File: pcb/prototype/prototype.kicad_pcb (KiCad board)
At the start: 2 copper layers, 39 parts, among them J1 GS2, J10 Conn_01x14, J11 Conn_01x14, J12 Conn_01x08, J13 Conn_01x08, J2 GS2, J3 GS2, J4 GS2, J5 GS2, J6 GS2, J7 GS2, J8 GS2, J9 Conn_01x14

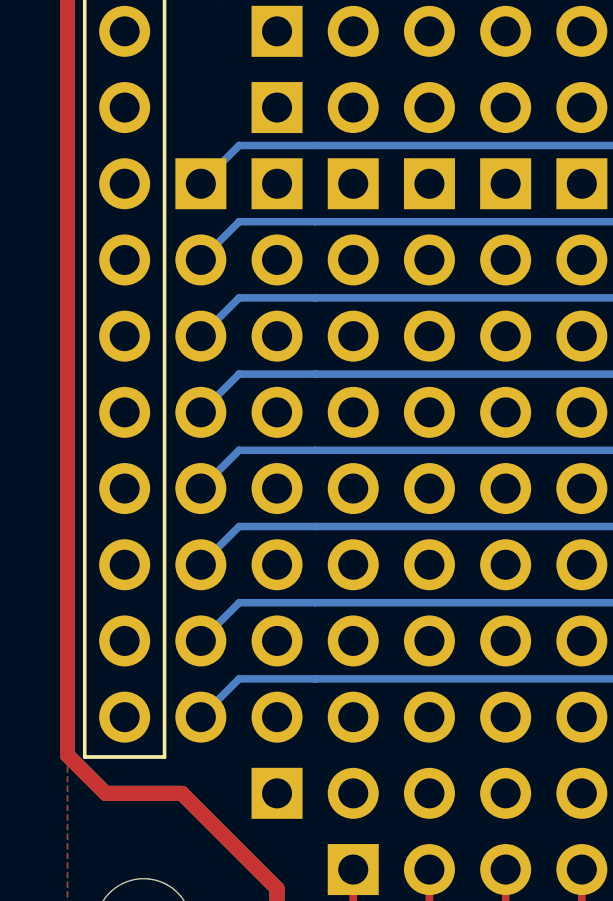
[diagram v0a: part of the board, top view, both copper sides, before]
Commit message: Ready for the second batch of PCBs to be printed.
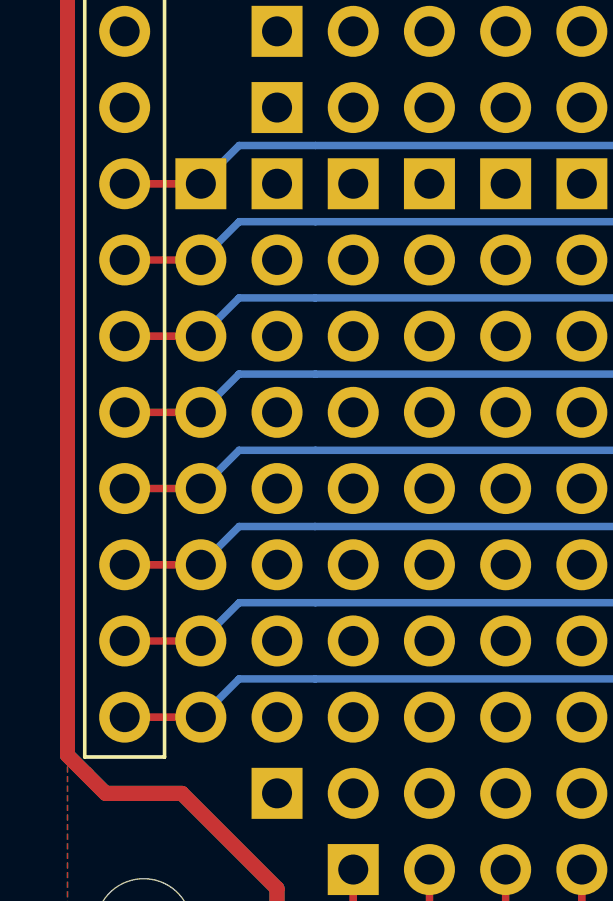
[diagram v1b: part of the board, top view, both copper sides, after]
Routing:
- net /L7: track 42.4 -> 45.0 mm
- net /L6: track 38.6 -> 41.2 mm
- net /L5: track 42.4 -> 45.0 mm
- net /L4: track 38.6 -> 41.2 mm
- net /L3: track 42.4 -> 45.0 mm
- net /L2: track 38.6 -> 41.2 mm
- net /L1: track 42.4 -> 45.0 mm
- net /L0: track 38.6 -> 41.2 mm
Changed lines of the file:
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@@
   (general
     (links 99)
-    (no_connects 8)
-    (area 123.19 81.915 172.720001 131.71)
+    (no_connects 0)
+    (area 123.19 81.915 172.720001 131.445001)
     (thickness 1.6)
     (drawings 15)
-    (tracks 151)
+    (tracks 159)
     (zones 0)
     (modules 39)
@@
   (segment (start 127 92.075) (end 128.905 90.17) (width 0.5) (layer F.Cu) (net 1))
   (segment (start 128.905 90.17) (end 131.445 90.17) (width 0.5) (layer F.Cu) (net 1))
+  (segment (start 126.365 102.87) (end 128.905 102.87) (width 0.25) (layer F.Cu) (net 3))
   (segment (start 167.005 101.595) (end 132.72 101.595) (width 0.25) (layer B.Cu) (net 3))
   (segment (start 132.72 101.595) (end 130.18 101.595) (width 0.25) (layer B.Cu) (net 3))
   (segment (start 130.18 101.595) (end 128.905 102.87) (width 0.25) (layer B.Cu) (net 3))
+  (segment (start 126.365 105.41) (end 128.905 105.41) (width 0.25) (layer F.Cu) (net 4))
   (segment (start 170.815 104.135) (end 132.72 104.135) (width 0.25) (layer B.Cu) (net 4))
   (segment (start 132.72 104.135) (end 130.18 104.135) (width 0.25) (layer B.Cu) (net 4))
   (segment (start 130.18 104.135) (end 128.905 105.41) (width 0.25) (layer B.Cu) (net 4))
+  (segment (start 126.365 107.95) (end 128.905 107.95) (width 0.25) (layer F.Cu) (net 5))
   (segment (start 132.715 106.675) (end 130.18 106.675) (width 0.25) (layer B.Cu) (net 5))
   (segment (start 130.18 106.675) (end 128.905 107.95) (width 0.25) (layer B.Cu) (net 5))
   (segment (start 167.005 106.675) (end 132.715 106.675) (width 0.25) (layer B.Cu) (net 5))
+  (segment (start 126.365 110.49) (end 128.905 110.49) (width 0.25) (layer F.Cu) (net 6))
   (segment (start 132.72 109.215) (end 130.18 109.215) (width 0.25) (layer B.Cu) (net 6))
   (segment (start 130.175 109.22) (end 128.905 110.49) (width 0.25) (layer B.Cu) (net 6))
   (segment (start 130.18 109.215) (end 130.175 109.22) (width 0.25) (layer B.Cu) (net 6))
   (segment (start 170.815 109.215) (end 132.72 109.215) (width 0.25) (layer B.Cu) (net 6))
+  (segment (start 126.365 113.03) (end 128.905 113.03) (width 0.25) (layer F.Cu) (net 7))
   (segment (start 132.72 111.755) (end 130.18 111.755) (width 0.25) (layer B.Cu) (net 7))
   (segment (start 130.18 111.755) (end 128.905 113.03) (width 0.25) (layer B.Cu) (net 7))
   (segment (start 167.005 111.755) (end 132.72 111.755) (width 0.25) (layer B.Cu) (net 7))
+  (segment (start 126.365 115.57) (end 128.905 115.57) (width 0.25) (layer F.Cu) (net 8))
   (segment (start 132.715 114.295) (end 130.18 114.295) (width 0.25) (layer B.Cu) (net 8))
   (segment (start 130.18 114.295) (end 128.905 115.57) (width 0.25) (layer B.Cu) (net 8))
   (segment (start 170.815 114.295) (end 132.715 114.295) (width 0.25) (layer B.Cu) (net 8))
+  (segment (start 126.365 118.11) (end 128.905 118.11) (width 0.25) (layer F.Cu) (net 9))
   (segment (start 132.72 116.835) (end 130.18 116.835) (width 0.25) (layer B.Cu) (net 9))
   (segment (start 130.18 116.835) (end 128.905 118.11) (width 0.25) (layer B.Cu) (net 9))
   (segment (start 167.005 116.835) (end 132.72 116.835) (width 0.25) (layer B.Cu) (net 9))
+  (segment (start 126.365 120.65) (end 128.905 120.65) (width 0.25) (layer F.Cu) (net 10))
   (segment (start 130.18 119.375) (end 128.905 120.65) (width 0.25) (layer B.Cu) (net 10))
   (segment (start 132.715 119.375) (end 130.18 119.375) (width 0.25) (layer B.Cu) (net 10))
